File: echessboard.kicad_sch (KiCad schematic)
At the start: 51 parts, among them J1 Conn_01x04_Pin, J3 USB_C_Receptacle_USB2.0_16P, J4 Conn_01x05_Pin, SW1 SW_Push, SW2 SW_Push, SW3 SW_Push, SW4 SW_Push, SW5 SW_Push, U1 STM32F030C6Tx, U3 USBLC6-2P6, U4 XC6206PxxxMR, U5 MCP2221AxST

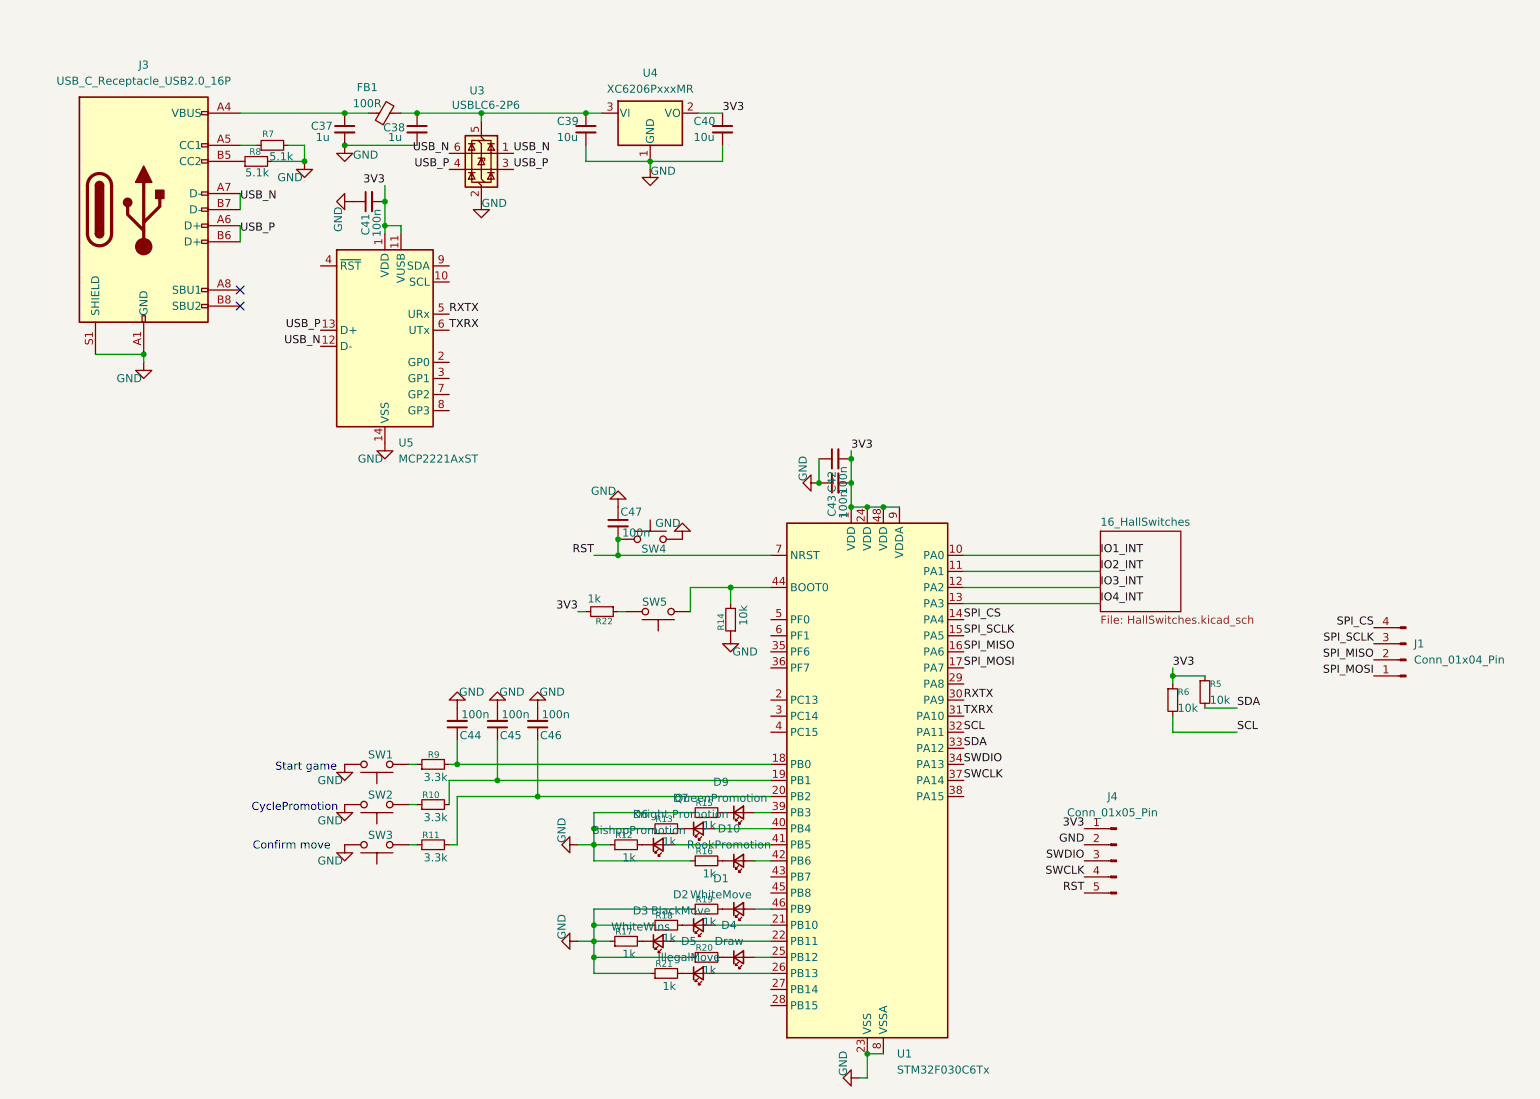
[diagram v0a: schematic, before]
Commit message: sync
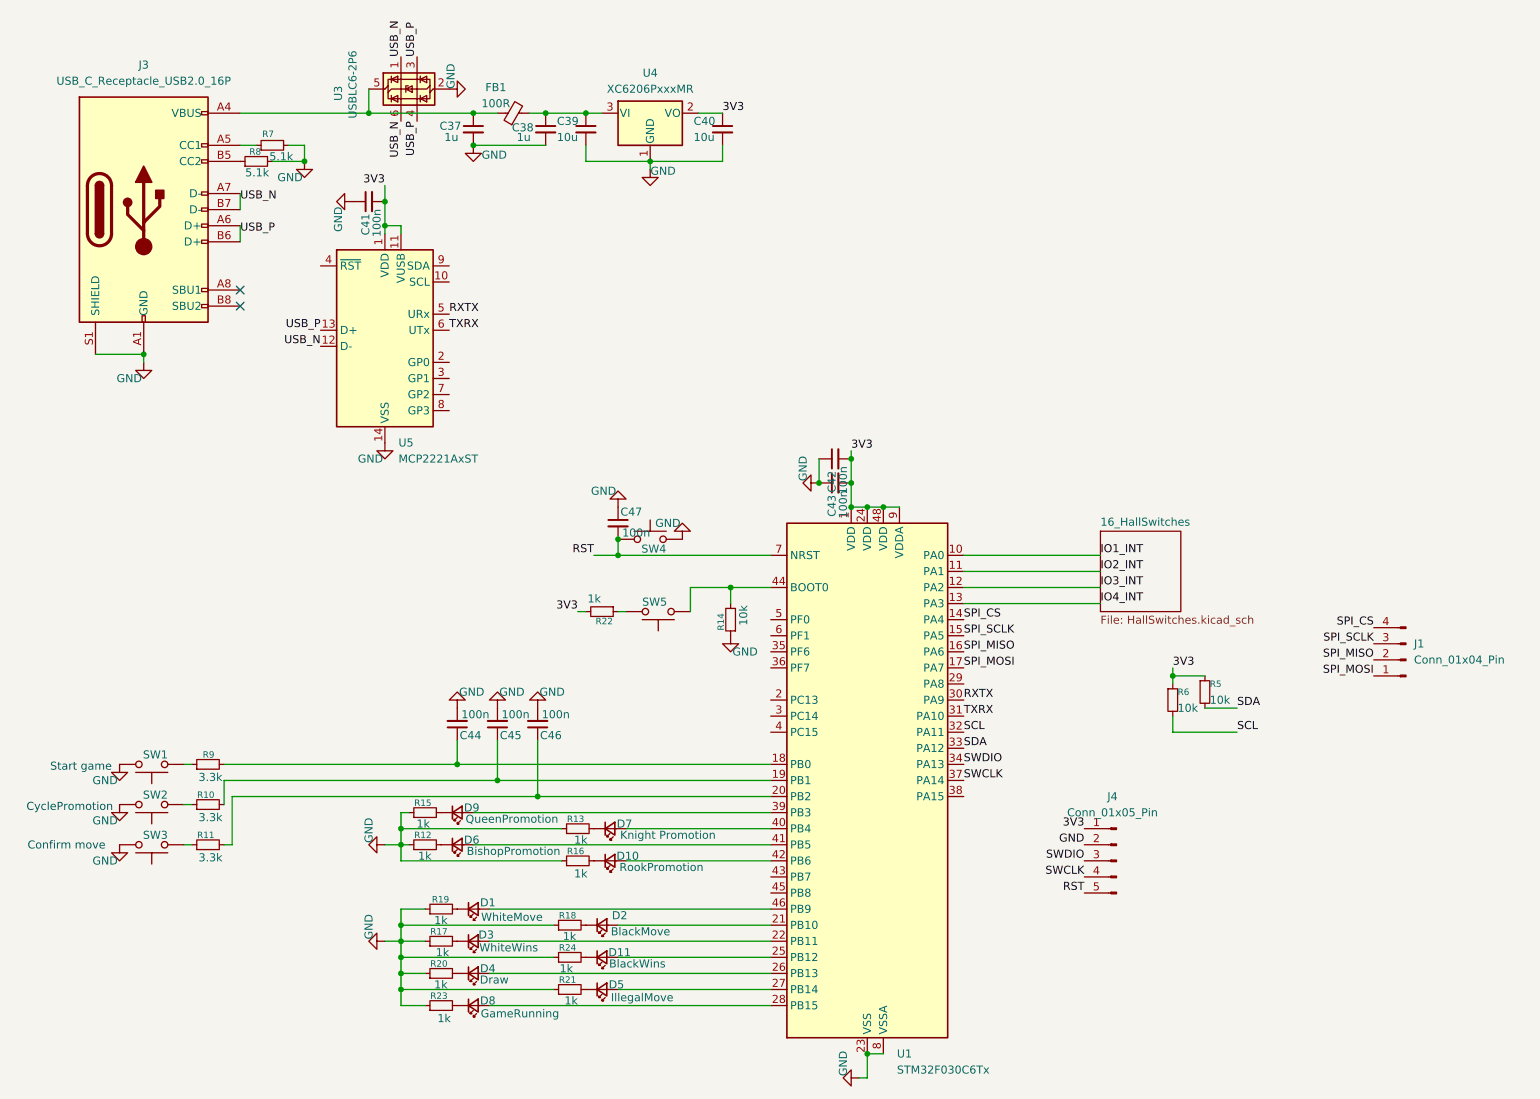
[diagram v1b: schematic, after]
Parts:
- added D11: BlackWins, LED_SMD:LED_0603_1608Metric, symbol Device:LED_Small
- added D8: GameRunning, LED_SMD:LED_0603_1608Metric, symbol Device:LED_Small
- added R23, R24: 1k, Resistor_SMD:R_0603_1608Metric, symbol Device:R_Small
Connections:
- net GND: now also R23.1, R24.1
- net at C38.1, C39.1, FB1.2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: no longer U3.5 (VBUS)
- net at C37.1, FB1.1, J3.A4 (VBUS)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: now also U3.5 (VBUS)
- net at U1.25 (PB12): now also D11.2 (A); no longer D4.2 (A)
- net at U1.26 (PB13): now also D4.2 (A); no longer D5.2 (A)
- net at U1.27 (PB14): now also D5.2 (A)
- net at U1.28 (PB15): now also D8.2 (A)
- new net: D8.1 (K), R23.2
- new net: D11.1 (K), R24.2
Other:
- moved on the sheet: C37, C38, D1, D10, D2, D3, D4, D5, D6, D7, D9, FB1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

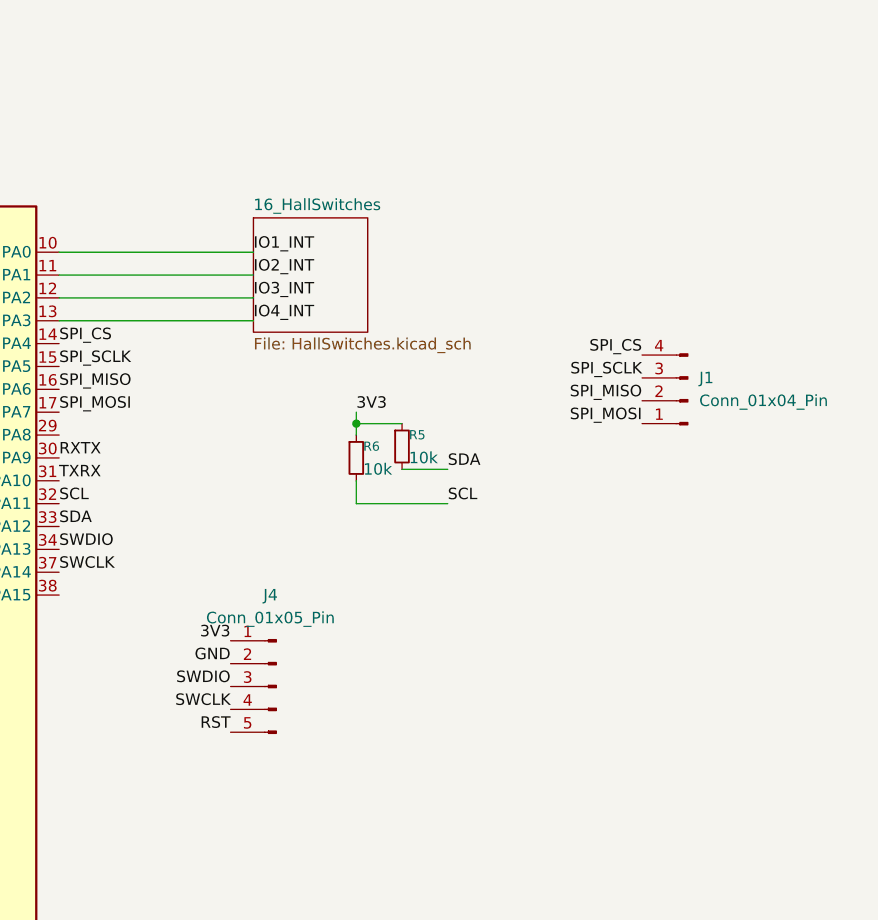
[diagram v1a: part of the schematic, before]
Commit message: sync
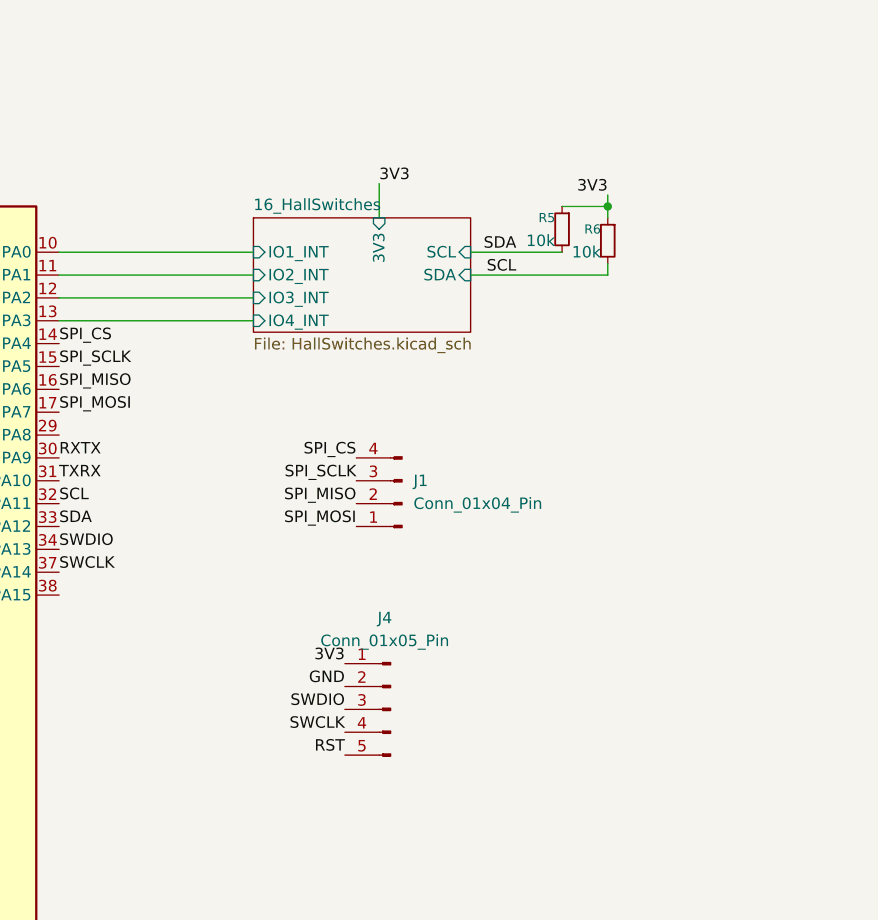
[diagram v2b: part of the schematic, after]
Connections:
- net IO1_INT renamed 16_HallSwitches/IO1_INT
- net IO2_INT renamed 16_HallSwitches/IO2_INT
- net IO3_INT renamed 16_HallSwitches/IO3_INT
- net IO4_INT renamed 16_HallSwitches/IO4_INT
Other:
- sheet 16_HallSwitches ports: added 3V3, IO1_INT, IO2_INT, IO3_INT, IO4_INT, SCL, SDA; removed none
- moved on the sheet: J1, J4, R5, R6
